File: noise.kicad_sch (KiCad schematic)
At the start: 10 parts, among them U34 74LS00, U36 74LS86, U57 74LS273, U58 74LS541, U59 4040, U60 74LS85, U61 74LS85, U62 74LS273, U63 74LS273, U64 74LS273

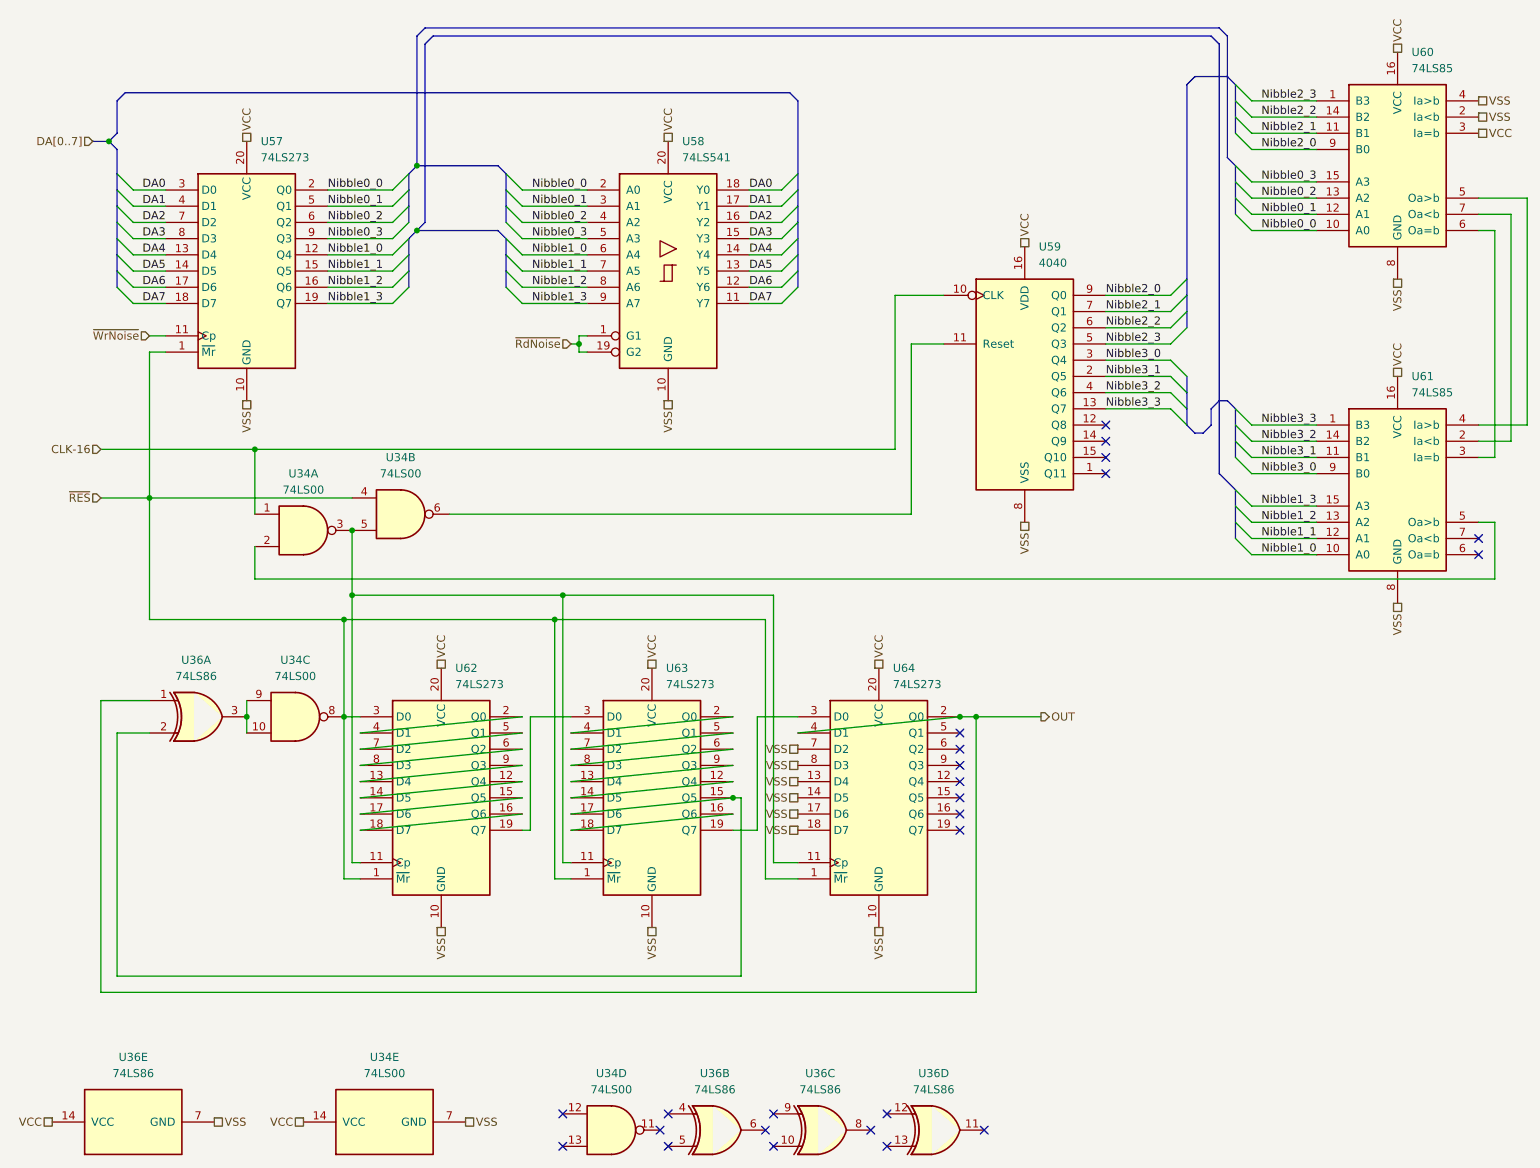
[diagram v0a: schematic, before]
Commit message: Fin de création de tous les schémas - envelope.kicad_sch - EnvelopeRate.kicad_sch
git-svn-id: file:///D%5C00%20-%20Dev%20&%20Calculs%5CRepoTortoiseSVN_PCB%5CRevivalChips/branches/Discrete-AY-3-8910@28 8d7748af-fe70-f644-8493-3f4b7ec62ef1
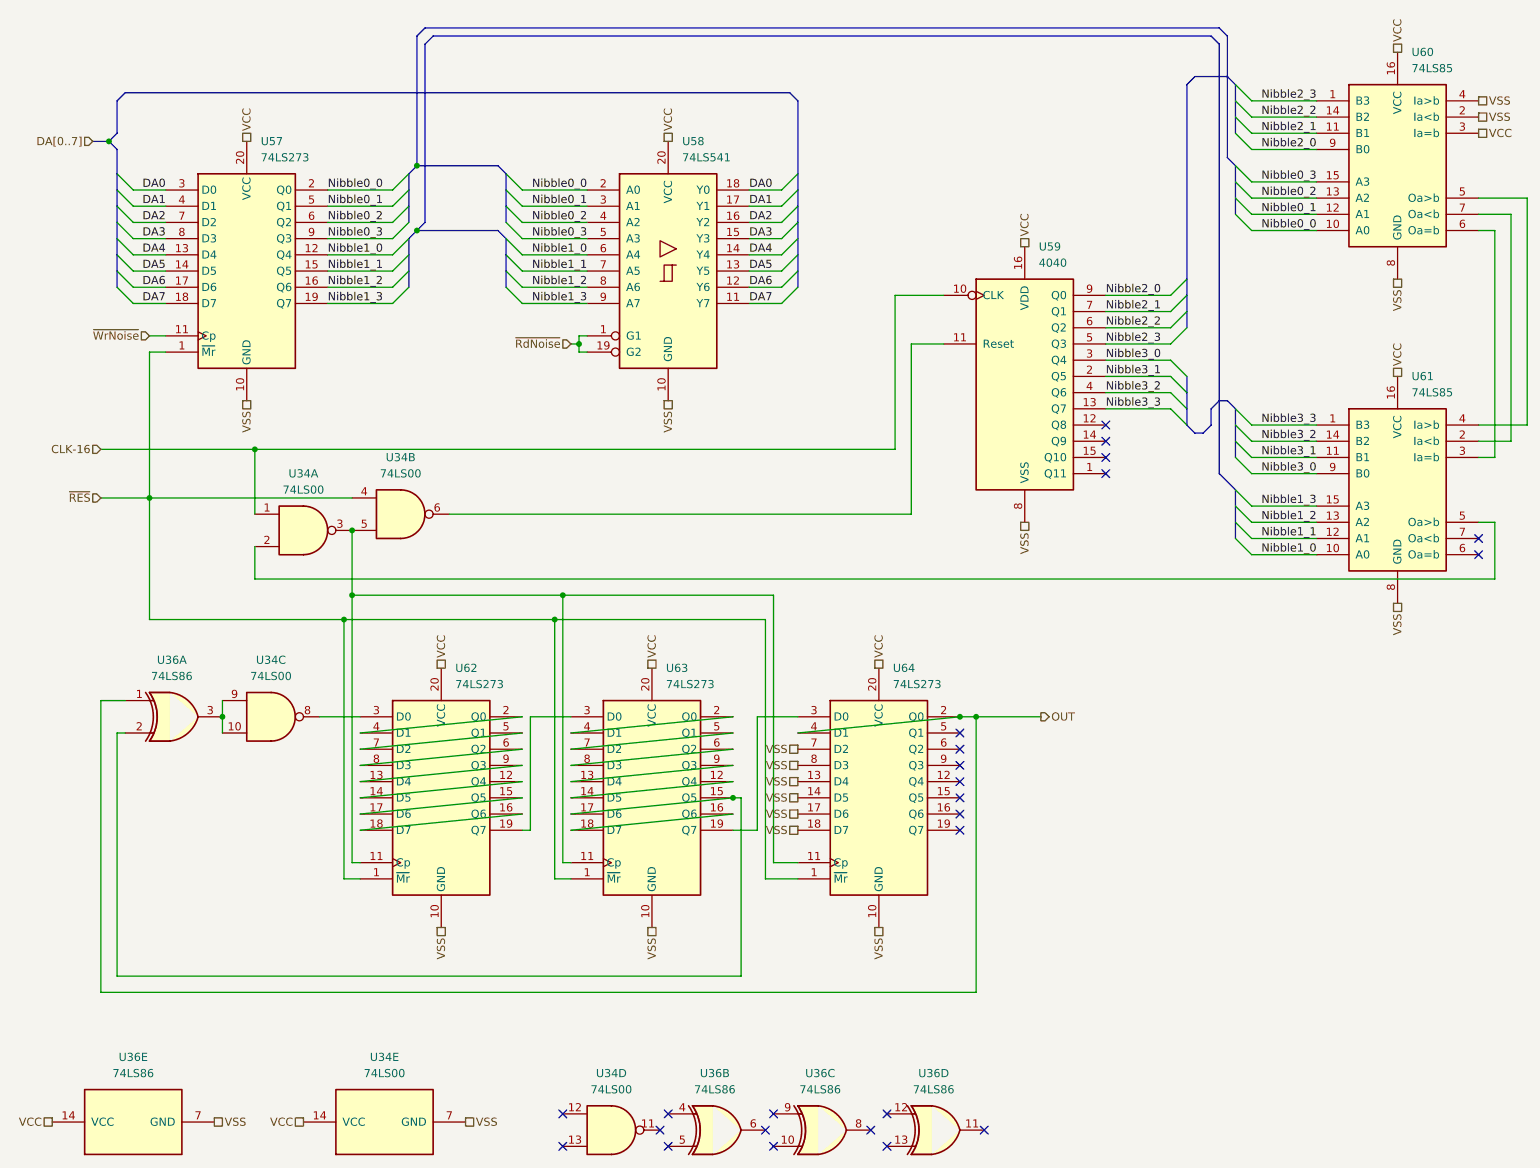
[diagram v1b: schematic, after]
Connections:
- net ~{RES}: no longer U34.8, U62.3 (D0)
- new net: U34.8, U62.3 (D0)
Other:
- moved on the sheet: U34C, U36A
